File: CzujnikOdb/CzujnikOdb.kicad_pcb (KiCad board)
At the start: 2 copper layers, 120 x 45.9 mm, 25 parts, among them J1 Conn_02x06_Odd_Even, U1 KTIR0711S, U2 KTIR0711S, U3 KTIR0711S, U4 KTIR0711S, U5 KTIR0711S, U6 KTIR0711S, U7 KTIR0711S, U8 KTIR0711S

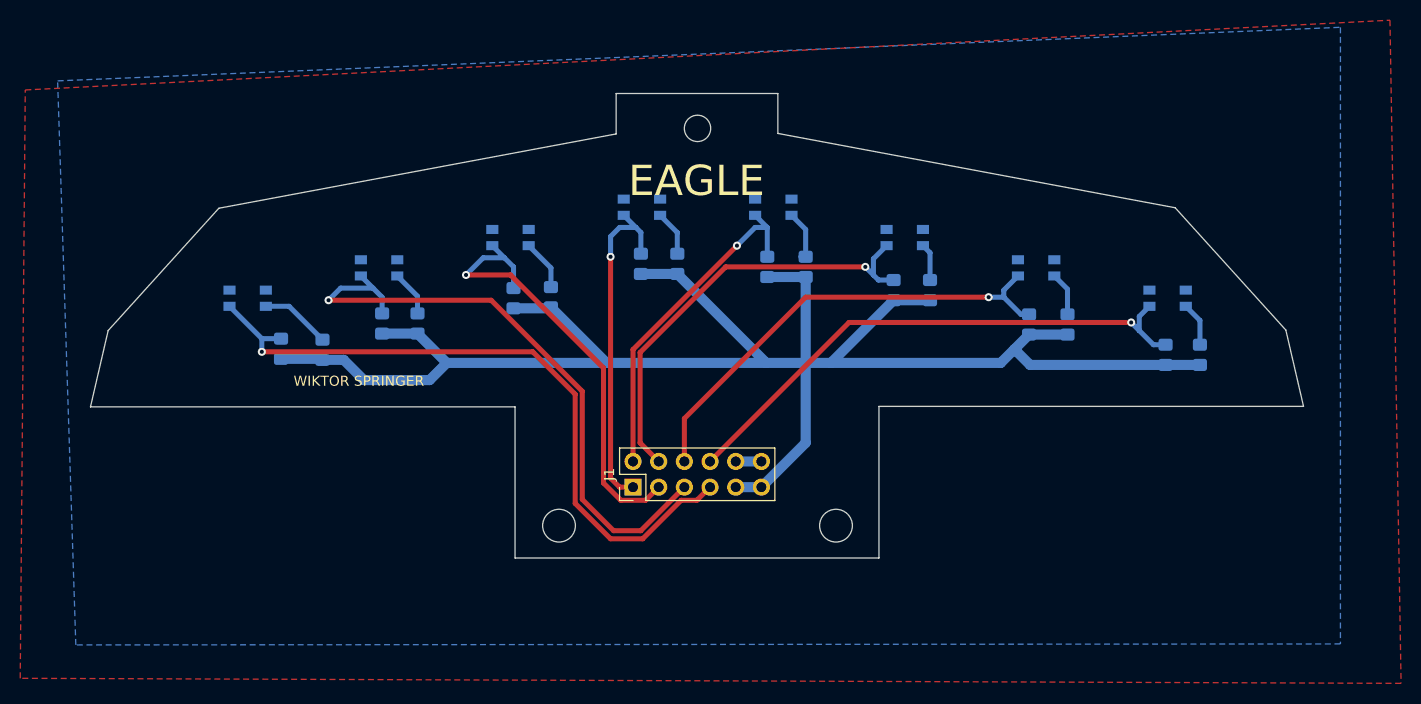
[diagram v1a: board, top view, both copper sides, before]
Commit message: Final version v2
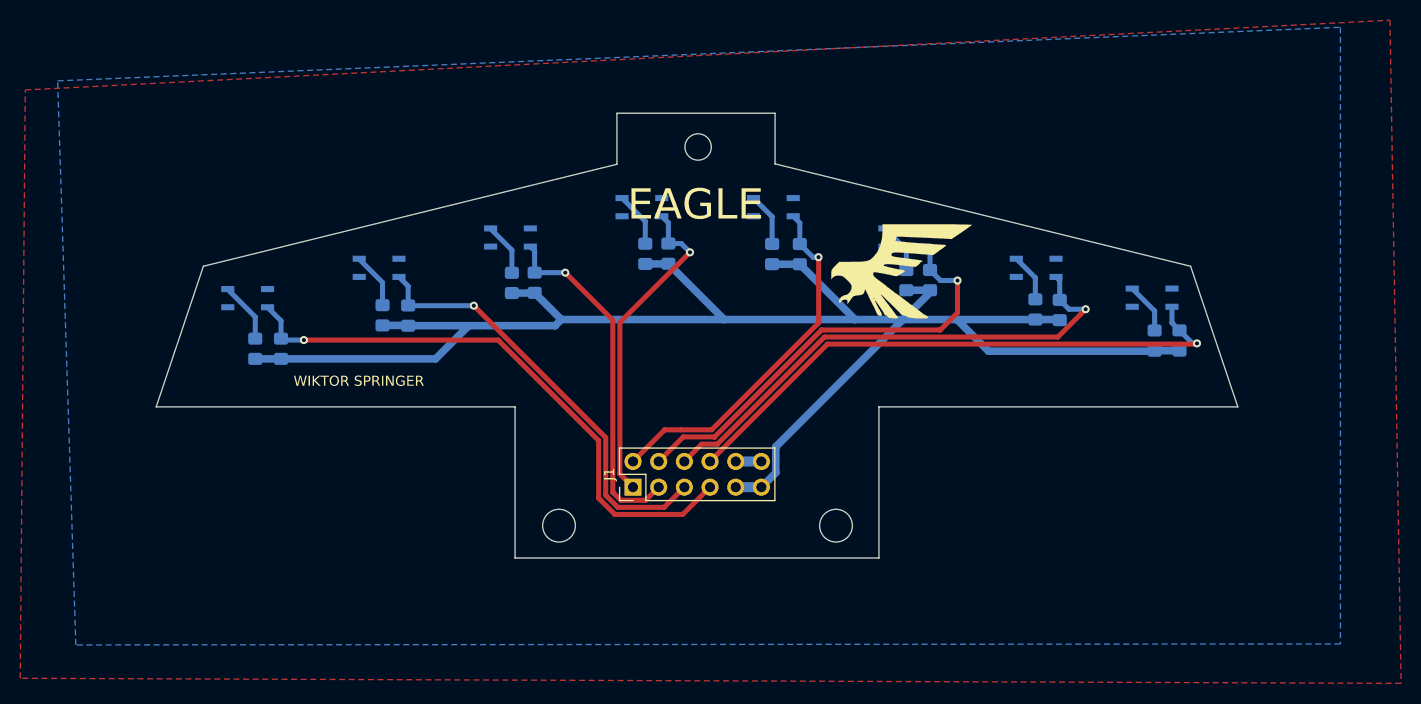
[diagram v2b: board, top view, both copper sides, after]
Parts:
- added G***: LOGO, warsztaty:log, F.Cu at (143.3, 105.4)
- U1, U2, U3, U4, U5, U6, U7, U8: footprint KTIR0711S:transoptor_KTIR0711S -> warsztaty:KTIR0711S
- moved R1 6.65 mm to (79.8, 112.5)
- moved R14 4.70 mm to (168.7, 111.7)
- moved R5 4.11 mm to (105.1, 106.0)
- moved R12 3.73 mm to (146.5, 105.7)
- moved R9 3.55 mm to (130.9, 103.1)
- moved R2 3.55 mm to (92.3, 109.2)
- moved R13 3.51 mm to (156.9, 108.6)
- moved R11 3.46 mm to (133.6, 103.1)
- moved R15 3.35 mm to (159.3, 108.7)
- moved R6 3.32 mm to (118.3, 103.1)
- moved R8 2.90 mm to (120.6, 103.1)
- moved R4 2.70 mm to (94.9, 109.2)
- moved R7 2.59 mm to (107.4, 106.0)
- moved R10 2.54 mm to (144.2, 105.7)
- moved R16 1.98 mm to (171.2, 111.7)
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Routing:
- net Out2: track 62.2 -> 43.0 mm
- net Out1: track 68.2 -> 57.8 mm
- net Out3: track 45.1 -> 34.9 mm
- net +3V3: track 176.0 -> 170.9 mm
- net Out7: track 46.7 -> 51.3 mm
- net Out8: track 54.5 -> 57.9 mm
- net Out5: track 34.0 -> 35.9 mm
- net Out4: track 33.9 -> 32.1 mm
- net Net-(R10-Pad2): track 3.69 -> 5.00 mm
- net Net-(R2-Pad2): track 4.53 -> 5.55 mm
- net Net-(R6-Pad2): track 4.50 -> 5.47 mm
- net Net-(R1-Pad2): track 6.97 -> 6.17 mm
- net Net-(R14-Pad2): track 4.38 -> 5.06 mm
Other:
- board size 120 x 45.9 mm -> 107 x 44 mm
